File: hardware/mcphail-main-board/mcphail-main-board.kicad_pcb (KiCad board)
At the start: 2 copper layers, 0 parts

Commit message: Release main board sch with BOM and layout estimates.
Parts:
- added B1: LIPO, Wickerlib:UNDEFINED, F.Cu at (147.2, 104.0)
- added BAT1: 3V, Wickerlib:BATT-HOLDER-CR1220-BK-916, F.Cu at (84.0, 84.6)
- added C10: 270nF, Wickerlib:RLC-0603-SMD, F.Cu at (114.1, 123.5)
- added C11: 1.5uF, Wickerlib:RLC-1206-SMD, F.Cu at (76.6, 138.8)
- added C12: 10nF, Wickerlib:RLC-0603-SMD, F.Cu at (125.1, 126.7)
- added C13: 1.5uF, Wickerlib:RLC-1206-SMD, F.Cu at (114.1, 113.3)
- added C14: 1uF, Wickerlib:RLC-0805-SMD, F.Cu at (121.9, 135.1)
- added C15: 22uF, Wickerlib:RLC-1210-SMD, F.Cu at (106.4, 127.3)
- added C16: 2.2uF, Wickerlib:RLC-1210-SMD, F.Cu at (114.1, 118.6)
- added C17: 2.2uF, Wickerlib:RLC-1210-SMD, F.Cu at (91.4, 141.8)
- added C18: 33pF, Wickerlib:RLC-0603-SMD, F.Cu at (110.8, 141.9)
- added C19: 2.2uF, Wickerlib:RLC-1210-SMD, F.Cu at (121.5, 113.8)
- added C2: DNP, Wickerlib:RLC-1206-SMD, F.Cu at (99.0, 129.7)
- added C20: 4.7uF, Wickerlib:RLC-1206-SMD, F.Cu at (106.7, 122.0)
- added C21: 4.7uF, Wickerlib:RLC-1206-SMD, F.Cu at (99.0, 124.9)
- added C22: 2.2uF, Wickerlib:RLC-1210-SMD, F.Cu at (105.9, 133.0)
- added C23: 4.7uF, Wickerlib:RLC-1206-SMD, F.Cu at (84.0, 138.8)
- added C24: 4.7uF, Wickerlib:RLC-1206-SMD, F.Cu at (82.2, 124.9)
- added C25: 10uF, Wickerlib:RLC-0805-SMD, F.Cu at (84.8, 143.5)
- added C26: 100nF, Wickerlib:RLC-0603-SMD, F.Cu at (119.2, 118.6)
- added C27: 22nF, Wickerlib:RLC-0603-SMD, F.Cu at (117.7, 135.6)
- added C28: 10nF, Wickerlib:RLC-0603-SMD, F.Cu at (120.8, 130.8)
- added C29: 1uF, Wickerlib:RLC-0805-SMD, F.Cu at (129.3, 127.9)
- added C3: 270nF, Wickerlib:RLC-0603-SMD, F.Cu at (96.5, 140.9)
- added C30: 100nF, Wickerlib:RLC-0603-SMD, F.Cu at (133.4, 83.4)
- added C31: 100nF, Wickerlib:RLC-0603-SMD, F.Cu at (111.0, 98.1)
- added C32: 100nF, Wickerlib:RLC-0603-SMD, F.Cu at (119.2, 92.7)
- added C33: 22pF, Wickerlib:RLC-0603-SMD, F.Cu at (132.9, 88.6)
- added C34: 1uF, Wickerlib:RLC-0805-SMD, F.Cu at (82.5, 106.1)
- added C35: 22pF, Wickerlib:RLC-0603-SMD, F.Cu at (120.8, 96.9)
- added C36: 100nF, Wickerlib:RLC-0603-SMD, F.Cu at (116.1, 98.1)
- added C37: 100nF, Wickerlib:RLC-0603-SMD, F.Cu at (113.1, 102.1)
- added C38: 100nF, Wickerlib:RLC-0603-SMD, F.Cu at (124.3, 92.9)
- added C39: 100nF, Wickerlib:RLC-0603-SMD, F.Cu at (104.5, 92.3)
- added C4: 1uF, Wickerlib:RLC-0805-SMD, F.Cu at (115.0, 140.5)
- added C40: 2pF, Wickerlib:RLC-0603-SMD, F.Cu at (95.3, 105.1)
- added C41: 100pF, Wickerlib:RLC-0603-SMD, F.Cu at (108.0, 103.0)
- added C42: 2pF, Wickerlib:RLC-0603-SMD, F.Cu at (117.4, 102.1)
- added C43: 4.7uF, Wickerlib:RLC-1206-SMD, F.Cu at (138.1, 120.5)
- added C44: 4.7uF, Wickerlib:RLC-1206-SMD, F.Cu at (106.7, 107.7)
- added C45: 4.7uF, Wickerlib:RLC-1206-SMD, F.Cu at (138.1, 125.3)
- added C46: 4.7uF, Wickerlib:RLC-1206-SMD, F.Cu at (132.8, 99.7)
- added C47: 100nF, Wickerlib:RLC-0603-SMD, F.Cu at (133.7, 104.1)
- added C48: 10pF, Wickerlib:RLC-0603-SMD, F.Cu at (139.8, 100.8)
- added C49: 1uF, Wickerlib:RLC-0805-SMD, F.Cu at (145.1, 97.1)
- added C5: 39nF, Wickerlib:RLC-0603-SMD, F.Cu at (128.4, 121.0)
- added C50: 1uF, Wickerlib:RLC-0805-SMD, F.Cu at (147.7, 127.6)
- added C6: 22uF, Wickerlib:RLC-1210-SMD, F.Cu at (99.0, 135.0)
- added C7: 1.5uF, Wickerlib:RLC-1206-SMD, F.Cu at (91.4, 136.5)
- added C8: 10nF, Wickerlib:RLC-0603-SMD, F.Cu at (124.9, 130.8)
- added C9: 1uF, Wickerlib:RLC-0805-SMD, F.Cu at (129.3, 125.3)
- added D1: 20V 1A, Wickerlib:DIODE-SMA, F.Cu at (89.8, 106.4)
- added D2: CG0603MLC-05E, Wickerlib:RLC-0603-SMD, F.Cu at (117.4, 88.6)
- added D3: CG0603MLC-05E, Wickerlib:RLC-0603-SMD, F.Cu at (95.3, 93.0)
- added D4: 20V 1A, Wickerlib:DIODE-SMA, F.Cu at (139.2, 143.7)
- added F1: 500mA, Wickerlib:RLC-1812-SMD, F.Cu at (127.4, 89.7)
- added J1: INSECT DETECTION, Wickerlib:CONN-HEADER-STRAIGHT-P2.54MM-1x02, F.Cu at (81.1, 132.8)
- added J2: EMITTERS, Wickerlib:CONN-HEADER-STRAIGHT-P2.54MM-1x02, F.Cu at (107.8, 116.0)
- added J3: BREAKOUT, Wickerlib:CONN-HEADER-STRAIGHT-P2.54MM-1x06, F.Cu at (77.6, 113.9)
- added J4: MICRO SD, Wickerlib:CONN-SD-MICRO-MOLEX-0475710001, F.Cu at (124.6, 71.3)
- added J5: MICRO USB, Wickerlib:CONN-USB-MICRO-B-AMPHENOL-10118193-0001LF, F.Cu at (103.1, 100.1)
- added J6: ISP, Wickerlib:CONN-HEADER-STRAIGHT-P2.54MM-2x03, F.Cu at (112.8, 79.6)
- added J7: FONA 808, Wickerlib:BREAKOUT-ADAFRUIT-FONA808-CELL-GPS, F.Cu at (95.9, 74.4)
- added J8: INPUT 6V-9V, Wickerlib:CONN-BARREL-JACK-2.5x5.5MM-TH, F.Cu at (144.9, 72.7)
- added J9: JST PH, Wickerlib:CONN-JST-S2B-PH-SM4-TB, F.Cu at (140.6, 134.6)
- added L1: FERRITE, Wickerlib:RLC-0402-SMD, F.Cu at (77.2, 105.7)
- added L2: 1uH 11A, Wickerlib:UNDEFINED, F.Cu at (146.4, 120.6)
- added LED1: AMBER, Wickerlib:LED-0603-SMD, F.Cu at (145.6, 123.3)
- added LED2: AMBER, Wickerlib:LED-0603-SMD, F.Cu at (128.4, 104.1)
- added LED3: AMBER, Wickerlib:LED-0603-SMD, F.Cu at (128.4, 108.2)
- added R1: 220, Wickerlib:RLC-0603-SMD, F.Cu at (114.6, 142.8)
- added R10: 732, Wickerlib:RLC-0603-SMD, F.Cu at (132.6, 134.3)
- added R11: 1.43K, Wickerlib:RLC-0603-SMD, F.Cu at (104.0, 137.9)
- added R12: 2.26K, Wickerlib:RLC-0603-SMD, F.Cu at (126.5, 112.9)
- added R13: 10K, Wickerlib:RLC-0603-SMD, F.Cu at (121.5, 137.4)
- added R14: 470, Wickerlib:RLC-0603-SMD, F.Cu at (125.0, 138.9)
- added R15: 97.6K, Wickerlib:RLC-0603-SMD, F.Cu at (110.9, 132.2)
- added R16: 2.26K, Wickerlib:RLC-0603-SMD, F.Cu at (111.4, 127.5)
- added R17: 68, Wickerlib:RLC-0603-SMD, F.Cu at (118.8, 141.4)
- added R18: 91K, Wickerlib:RLC-0603-SMD, F.Cu at (125.7, 134.8)
- added R19: 91K, Wickerlib:RLC-0603-SMD, F.Cu at (128.9, 130.2)
- added R2: 64.9K, Wickerlib:RLC-0603-SMD, F.Cu at (131.3, 112.9)
- added R20: 200K, Wickerlib:RLC-0805-SMD, F.Cu at (80.5, 143.5)
- added R21: 200K, Wickerlib:RLC-0805-SMD, F.Cu at (76.2, 143.5)
- added R22: 2.2K, Wickerlib:RLC-0603-SMD, F.Cu at (132.5, 121.0)
- added R23: 2.26K, Wickerlib:RLC-0603-SMD, F.Cu at (116.3, 127.5)
- added R24: 22K, Wickerlib:RLC-0603-SMD, F.Cu at (132.4, 130.2)
- added R25: 4.32K, Wickerlib:RLC-0603-SMD, F.Cu at (123.9, 122.7)
- added R26: 2.2K, Wickerlib:RLC-0603-SMD, F.Cu at (122.5, 142.9)
- added R27: 2.94K, Wickerlib:RLC-0603-SMD, F.Cu at (115.8, 131.6)
- added R28: 22K, Wickerlib:RLC-0603-SMD, F.Cu at (129.1, 138.3)
- added R29: 4.32K, Wickerlib:RLC-0603-SMD, F.Cu at (108.8, 137.9)
- added R3: 100K, Wickerlib:RLC-0603-SMD, F.Cu at (120.9, 126.7)
- added R30: 3.83K, Wickerlib:RLC-0603-SMD, F.Cu at (126.5, 117.0)
- added R31: 22, Wickerlib:RLC-0603-SMD, F.Cu at (120.8, 101.0)
- added R32: 22, Wickerlib:RLC-0603-SMD, F.Cu at (136.7, 87.5)
- added R33: 10K, Wickerlib:RLC-0603-SMD, F.Cu at (128.0, 96.9)
- added R34: 2K, Wickerlib:RLC-0603-SMD, F.Cu at (132.5, 92.7)
- added R35: 2K, Wickerlib:RLC-0603-SMD, F.Cu at (124.6, 96.9)
- added R36: 10K, Wickerlib:RLC-0603-SMD, F.Cu at (128.6, 92.9)
- added R37: 1K, Wickerlib:RLC-0603-SMD, F.Cu at (137.7, 83.4)
- added R38: 0 ohm, Wickerlib:RLC-0603-SMD, F.Cu at (140.4, 96.8)
- added R39: 470, Wickerlib:RLC-0603-SMD, F.Cu at (143.6, 103.5)
- added R4: 100K, Wickerlib:RLC-0603-SMD, F.Cu at (113.5, 136.2)
- added R40: 470, Wickerlib:RLC-0603-SMD, F.Cu at (137.2, 108.9)
- added R41: 470, Wickerlib:RLC-0603-SMD, F.Cu at (137.9, 104.9)
- added R42: NTC 10K, Wickerlib:RLC-0402-SMD, F.Cu at (111.1, 107.8)
- added R43: 2K, Wickerlib:RLC-0603-SMD, F.Cu at (144.8, 99.5)
- added R44: 100K, Wickerlib:RLC-0603-SMD, F.Cu at (150.5, 123.2)
- added R45: 1M, Wickerlib:RLC-0603-SMD, F.Cu at (148.2, 99.5)
- added R46: 111K, Wickerlib:RLC-0603-SMD, F.Cu at (133.3, 108.2)
- added R47: 1M, Wickerlib:RLC-0603-SMD, F.Cu at (141.4, 107.6)
- added R5: 1.87K, Wickerlib:RLC-0603-SMD, F.Cu at (101.5, 141.9)
- added R6: 3.83K, Wickerlib:RLC-0603-SMD, F.Cu at (119.1, 122.7)
- added R7: 10, Wickerlib:RLC-0603-SMD, F.Cu at (129.1, 134.3)
- added R8: 1.43K, Wickerlib:RLC-0603-SMD, F.Cu at (131.3, 117.0)
- added R9: 1.02K, Wickerlib:RLC-0603-SMD, F.Cu at (106.3, 141.9)
- added S1: RESET, Wickerlib:SWITCH-OMRON-MOMENTARY-SMD-B3U-1000P, F.Cu at (109.5, 93.5)
- added U1: MCP6004, Wickerlib:SOIC-14-3.9x8.7MM-P1.27MM, F.Cu at (83.7, 117.0)
- added U10: BUCK-BOOST 5V TPS63060, Wickerlib:QFN-20-1EP-4x4MM_P0.5MM, F.Cu at (145.4, 92.4)
- added U11: MCP1703, Wickerlib:SOT-23-3, F.Cu at (118.4, 105.7)
- added U2: MCP6004, Wickerlib:SOIC-14-3.9x8.7MM-P1.27MM, F.Cu at (91.9, 117.0)
- added U3: TLV274, Wickerlib:SOIC-14-3.9x8.7MM-P1.27MM, F.Cu at (100.0, 117.0)
- added U4: MCP6004, Wickerlib:SOIC-14-3.9x8.7MM-P1.27MM, F.Cu at (92.4, 128.5)
- added U5: TXB0104, Wickerlib:SOIC-14-3.9x8.7MM-P1.27MM, F.Cu at (134.9, 75.9)
- added U6: ATMEGA32U4-TQFP44, Wickerlib:TQFP-44-10x10MM-P0.8MM, F.Cu at (102.4, 84.3)
- added U7: 24AA1025 EEPROM, Wickerlib:SOIC-8-3.9x4.9MM-P1.27MM, F.Cu at (81.3, 95.4)
- added U8: MCP7940N RTC, Wickerlib:SOIC-8-3.9x4.9MM-P1.27MM, F.Cu at (80.0, 101.8)
- added U9: MCP73871, Wickerlib:QFN-20-1EP-4x4MM_P0.5MM, F.Cu at (140.3, 115.8)
- added W1: TEST_1P, Wickerlib:HOLE-PLATED-40MIL, F.Cu at (134.1, 139.6)
- added X1: 16MHz, Wickerlib:CRYSTAL-CTS-4SMD, F.Cu at (101.6, 104.8)
- added X2: 32.768kHz, Wickerlib:CRYSTAL-HC49-TH, F.Cu at (91.9, 101.2)
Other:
- board outline added: 78.7 x 78.7 mm
- rule trace_clearance: 0.1524 -> 0.254

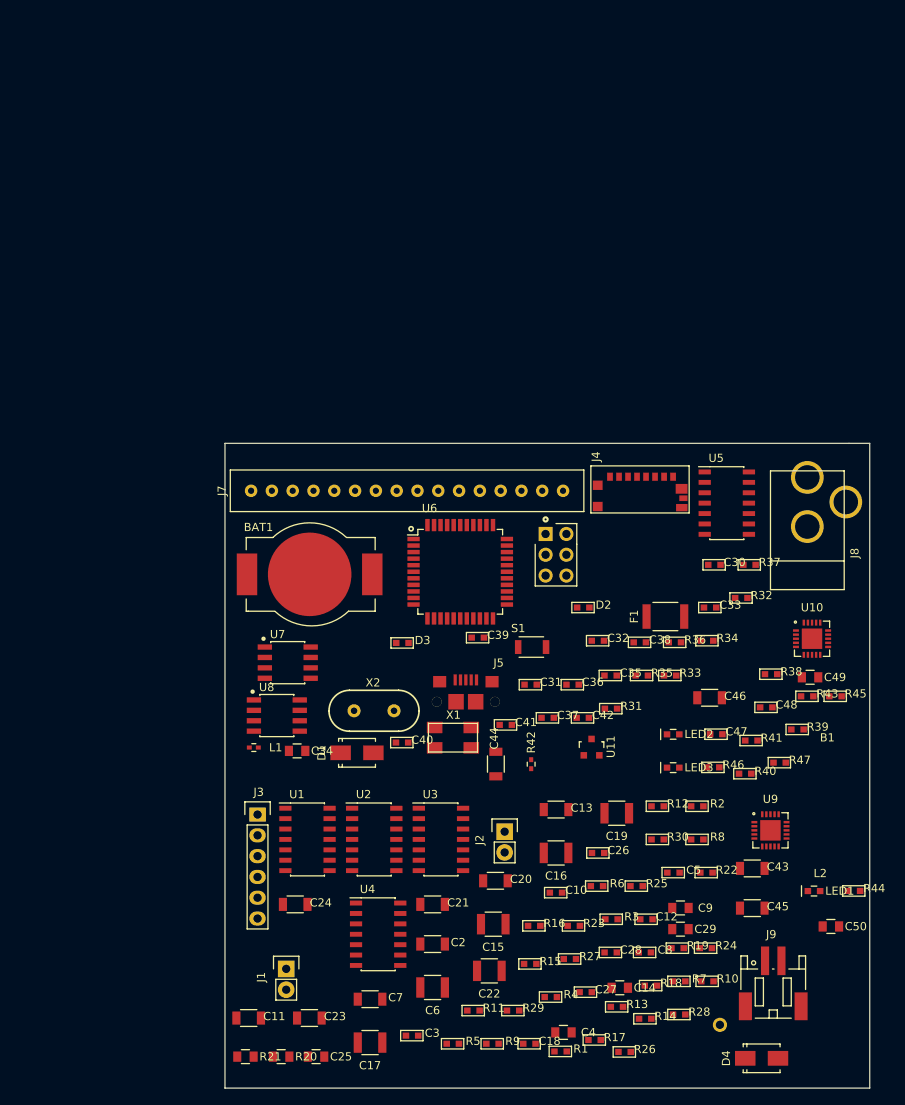
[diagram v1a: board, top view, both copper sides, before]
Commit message: Hooked up pins to ATSAMD21G18 Cortex M0, fixed AGND throughout.
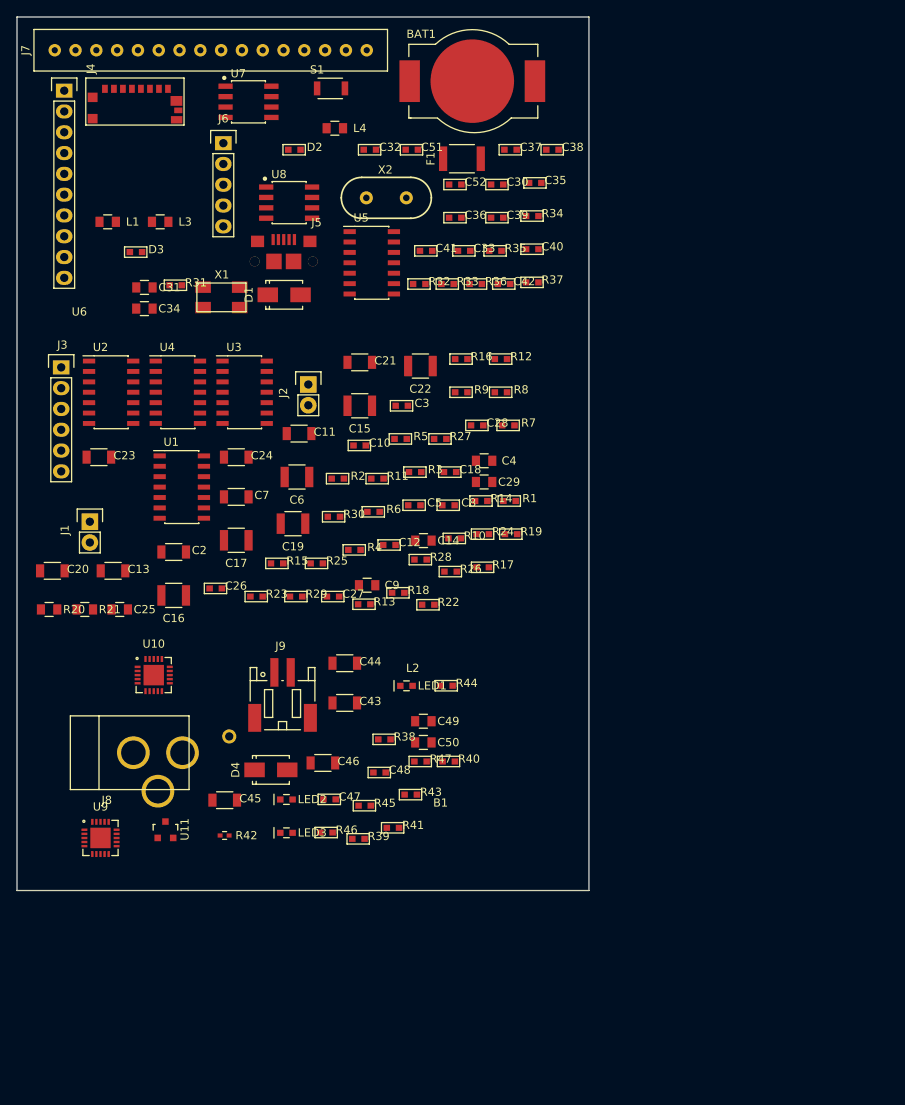
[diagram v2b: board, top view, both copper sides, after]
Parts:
- added C51: 100nF, Wickerlib:RLC-0603-SMD, F.Cu at (96.5, 32.7)
- added C52: 100nF, Wickerlib:RLC-0603-SMD, F.Cu at (101.8, 37.0)
- added J10: BREAKOUT, Wickerlib:CONN-HEADER-STRAIGHT-P2.54MM-1x10, F.Cu at (54.0, 25.5)
- added L3: FERRITE, Wickerlib:RLC-0805-SMD, F.Cu at (65.7, 41.5)
- added L4: FERRITE, Wickerlib:RLC-0805-SMD, F.Cu at (87.1, 30.1)
- C31: value 100nF -> 10uF; footprint Wickerlib:RLC-0603-SMD -> Wickerlib:RLC-0805-SMD
- J6: value ISP -> SWD; footprint Wickerlib:CONN-HEADER-STRAIGHT-P2.54MM-2x03 -> Wickerlib:CONN-HEADER-STRAIGHT-P2.54MM-1x05
- L1: footprint Wickerlib:RLC-0402-SMD -> Wickerlib:RLC-0805-SMD
- R31: value 22 -> 330
- R32: value 22 -> 1K
- U5: value TXB0104 -> ADS1118
- U6: value ATMEGA32U4-TQFP44 -> ATSAMD21G18A; footprint Wickerlib:TQFP-44-10x10MM-P0.8MM -> Wickerlib:UNDEFINED
- moved J8 83.5 mm to (68.5, 106.5), turned to 0 degrees
- moved U9 81.8 mm to (58.5, 116.8)
- moved U10 80.5 mm to (65.0, 96.9)
- moved R9 79.7 mm to (102.5, 62.3)
- moved J4 77.8 mm to (62.9, 24.0)
- moved C3 76.9 mm to (95.3, 64.0)
- moved C22 74.3 mm to (97.5, 59.1)
- moved R31 74.2 mm to (67.6, 49.3)
- moved R5 74.1 mm to (95.1, 68.0)
- moved C23 73.2 mm to (58.3, 70.3)
- moved S1 72.5 mm to (84.9, 25.2)
- moved C11 71.6 mm to (82.7, 67.4)
- moved R7 71.0 mm to (108.3, 66.4)
- moved U4 70.6 mm to (67.9, 62.3)
- moved C4 70.5 mm to (105.3, 70.7)
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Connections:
- C14 pad 2: GND -> AGND
- C29 pad 2: GND -> AGND
- C31 pad 1: +5V -> /Microcontroller/VDDANA
- C31 pad 2: GND -> AGND
- C34 pad 1: /Microcontroller/VUSB_IN -> (no net)
- C36 pad 1: +5V -> +3V3
- C37 pad 1: +5V -> +3V3
- C38 pad 1: +5V -> +3V3
- C39 pad 1: +5V -> +3V3
- C4 pad 2: GND -> AGND
- C6 pad 2: GND -> AGND
- C9 pad 2: GND -> AGND
- D2 pad 1: Net-(D2-Pad1) -> /Microcontroller/USB_D-
- D3 pad 1: Net-(D3-Pad1) -> /Microcontroller/USB_D+
- F1 pad 1: /Microcontroller/VUSB_IN -> Net-(D1-Pad2)
- F1 pad 2: Net-(D1-Pad2) -> /Microcontroller/VUSB_IN
- J3 pad 6: GND -> AGND
- J4 pad 2: /Microcontroller/SD_CS -> /Microcontroller/D4_CS
- J4 pad 3: /Microcontroller/SD_MOSI -> /Microcontroller/MOSI
- J4 pad 5: /Microcontroller/SD_SCLK -> /Microcontroller/SCLK
- J4 pad 7: /Microcontroller/SD_MISO -> /Microcontroller/MISO
- J5 pad 1: Net-(D1-Pad2) -> /Microcontroller/VUSB_IN
- J5 pad 2: Net-(D2-Pad1) -> /Microcontroller/USB_D-
- J5 pad 3: Net-(D3-Pad1) -> /Microcontroller/USB_D+
- J5 pad 4: /Microcontroller/USB_GND -> (no net)
- J5 pad 5: /Microcontroller/USB_GND -> Net-(J5-Pad5)
- J6 pad 1: /Microcontroller/MISO -> +3V3
- J6 pad 2: +5V -> (no net)
- J6 pad 3: /Microcontroller/SCLK -> /Microcontroller/SWCLK
- J6 pad 4: /Microcontroller/MOSI -> /Microcontroller/~RESET
- J6 pad 5: /Microcontroller/~RESET -> GND
- J7 pad 10: /Microcontroller/FONA_RI -> (no net)
- J7 pad 11: /Microcontroller/FONA_PS -> (no net)
- J7 pad 12: /Microcontroller/FONA_NS -> (no net)
- J7 pad 4: +5V -> +3V3
- J7 pad 5: /Microcontroller/FONA_RST -> (no net)
- J7 pad 6: /Microcontroller/FONA_RX -> (no net)
- J7 pad 7: /Microcontroller/FONA_TX -> (no net)
- J7 pad 8: /Microcontroller/FONA_RTS -> (no net)
- L1 pad 1: /Microcontroller/USB_GND -> Net-(J5-Pad5)
- R19 pad 2: GND -> AGND
- R31 pad 1: /Microcontroller/USB_D- -> /Microcontroller/~RESET
- R31 pad 2: Net-(D2-Pad1) -> Net-(R31-Pad2)
- R32 pad 1: /Microcontroller/USB_D+ -> +3V3
- R32 pad 2: Net-(D3-Pad1) -> /Microcontroller/SWCLK
- R33 pad 1: +5V -> +3V3
- R34 pad 1: +5V -> +3V3
- R35 pad 1: +5V -> +3V3
- R36 pad 1: +5V -> +3V3
- R4 pad 2: GND -> AGND
- S1 pad 1: /Microcontroller/~RESET -> Net-(R31-Pad2)
- U1 pad 11: GND -> AGND
- U2 pad 11: GND -> AGND
- U3 pad 11: GND -> AGND
- U4 pad 11: GND -> AGND
- U5 pad 1: +3V3 -> /Microcontroller/SCLK
- U5 pad 10: /Microcontroller/D4_CS -> /Microcontroller/MOSI
- U5 pad 11: /Microcontroller/SCLK -> (no net)
- U5 pad 12: /Microcontroller/MOSI -> (no net)
- U5 pad 13: /Microcontroller/MISO -> (no net)
- U5 pad 14: +5V -> (no net)
- U5 pad 2: /Microcontroller/SD_MISO -> /Microcontroller/D4_CS
- U5 pad 3: /Microcontroller/SD_MOSI -> GND
- U5 pad 4: /Microcontroller/SD_SCLK -> /A0
- U5 pad 5: /Microcontroller/SD_CS -> /A1
- U5 pad 6: (no net) -> /A2
- U5 pad 7: GND -> +3V3
- U5 pad 9: (no net) -> /Microcontroller/MISO
- U7 pad 1: /Microcontroller/EEPROM_A0 -> (no net)
- U7 pad 2: /Microcontroller/EEPROM_A1 -> (no net)
- U7 pad 3: /Microcontroller/EEPROM_A2 -> (no net)
- U7 pad 8: +5V -> +3V3
- U8 pad 8: +5V -> +3V3
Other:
- board size 78.7 x 78.7 mm -> 69.8 x 106.7 mm
